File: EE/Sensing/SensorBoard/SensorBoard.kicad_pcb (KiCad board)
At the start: 2 copper layers, 40 x 76.5 mm, 123 parts, among them J1 Conn_01x04_Male, J101 Peg, J102 Peg, J11 Peg, J12 Peg, J21 Peg, J22 Peg, J31 Peg, J32 Peg, J41 Peg, J42 Peg, J51 Peg, J52 Peg, J61 Peg, J62 Peg, J71 Peg, J72 Peg, J81 Peg, J82 Peg, J91 Peg, J92 Peg, Q1 BSS84DW, Q10 BSS84DW, Q11 DMP31D1U-7, Q12 DMP31D1U-7, Q2 BSS84DW, Q3 BSS84DW, Q4 BSS84DW, Q5 BSS84DW, Q6 BSS84DW, Q7 BSS84DW, Q8 BSS84DW, Q9 BSS84DW, U1 TCR2EE27, U101 AH1381, U102 AH1381, U11 AH1381, U12 AH1381, U2 TCR2EE32, U21 AH1381, U22 AH1381, U3 TCA9555PWR, U31 AH1381, U32 AH1381, U41 AH1381, U42 AH1381, U51 AH1381, U52 AH1381, U61 AH1381, U62 AH1381, U71 AH1381, U72 AH1381, U81 AH1381, U82 AH1381, U91 AH1381, U92 AH1381

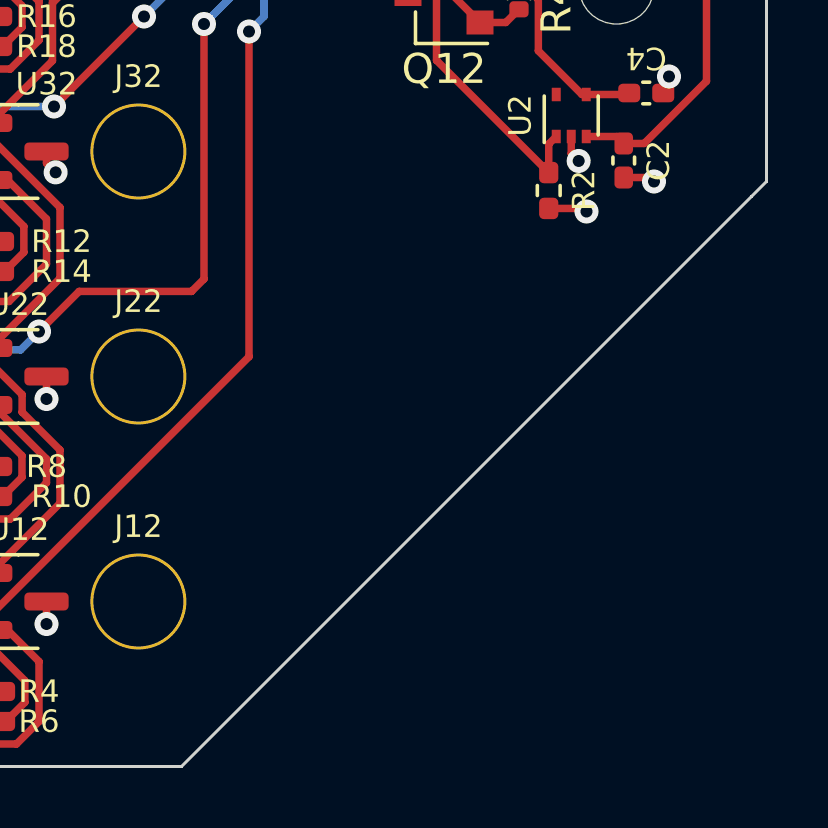
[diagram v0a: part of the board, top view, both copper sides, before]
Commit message: Updated layout, and placement for main board
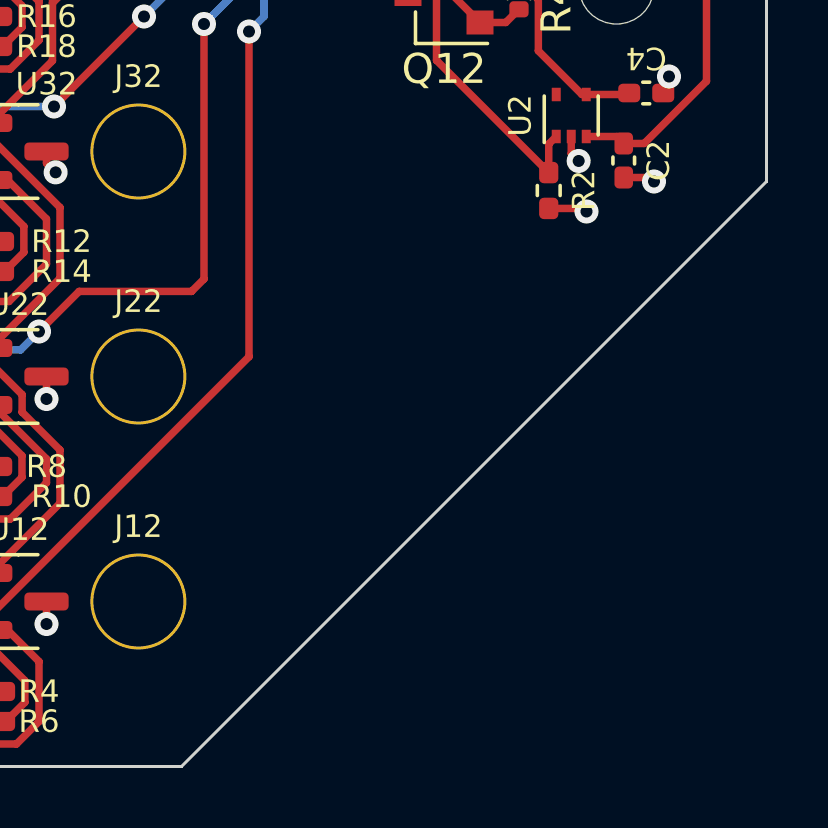
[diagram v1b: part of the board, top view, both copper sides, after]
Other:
- outline, holes or cut-outs redrawn
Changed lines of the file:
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@@
   (gr_line (start 218 48.5) (end 218 35.5) (layer "Edge.Cuts") (width 0.1))
   (gr_line (start 218 95.5) (end 218 75.5) (layer "Edge.Cuts") (width 0.1))
-  (gr_line (start 238.5 95.5) (end 257.5 76.5) (layer "Edge.Cuts") (width 0.1))
+  (gr_line (start 238.5 95.5) (end 258 76) (layer "Edge.Cuts") (width 0.1))
   (gr_line (start 234.5 95.5) (end 238 95.5) (layer "Edge.Cuts") (width 0.1))
   (gr_line (start 258 38) (end 239 19) (layer "Edge.Cuts") (width 0.1))
-  (gr_line (start 258 76) (end 257.5 76.5) (layer "Edge.Cuts") (width 0.1))
   (gr_line (start 238 95.5) (end 238.5 95.5) (layer "Edge.Cuts") (width 0.1))
   (gr_line (start 218 48.5) (end 218 62.5) (layer "Edge.Cuts") (width 0.1))
